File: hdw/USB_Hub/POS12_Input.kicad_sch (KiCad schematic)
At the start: 21 parts

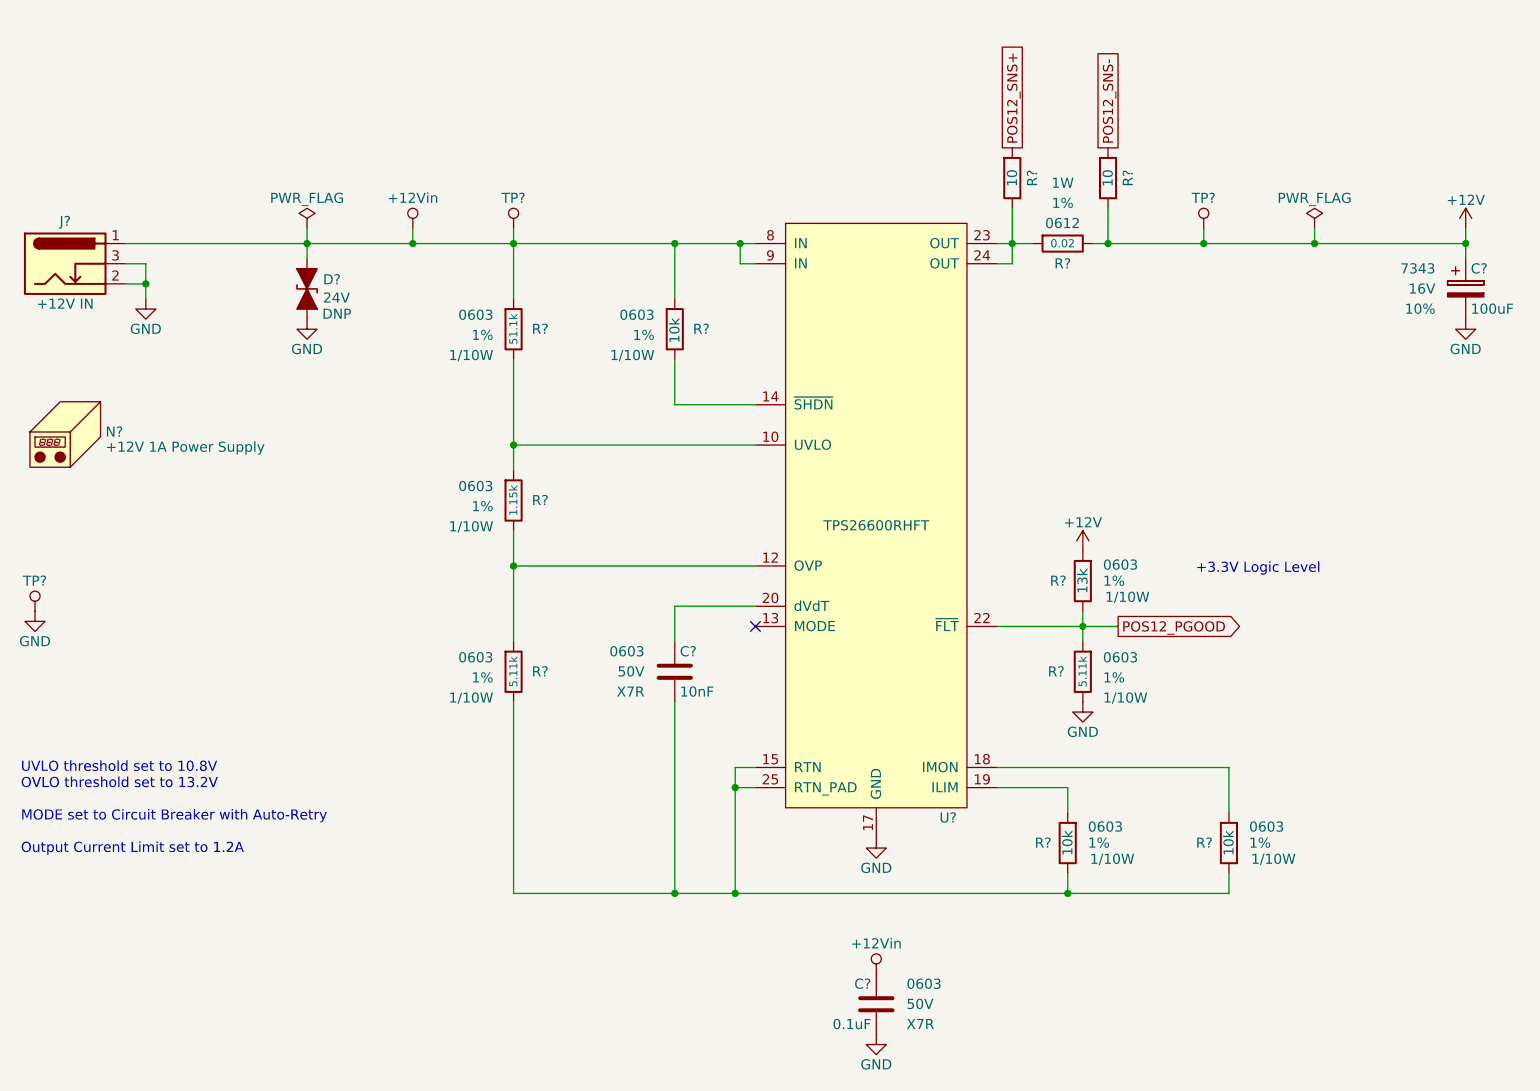
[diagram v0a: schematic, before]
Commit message: big restructuring, removed microcontroller and all telemtry
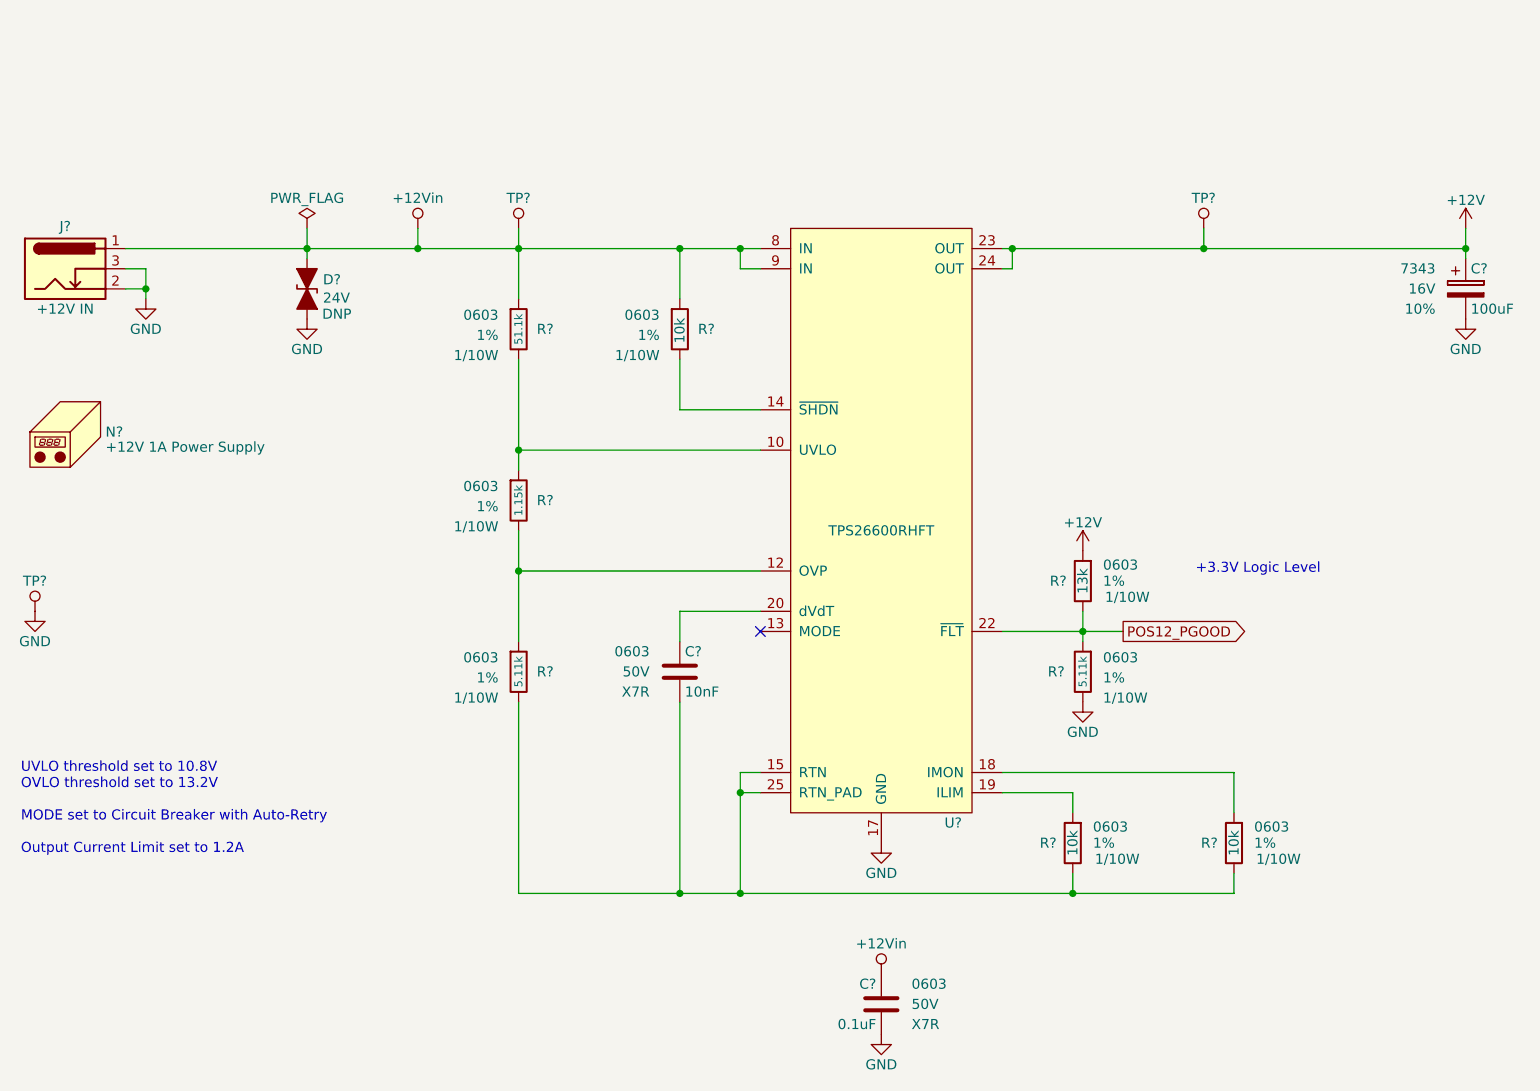
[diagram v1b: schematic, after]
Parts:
- removed R? (x2): 10, Resistors_SMD:R_0603, symbol Custom_Library:R_Custom
- removed R?: 0.02, Resistors_SMD:R_0612, symbol Custom_Library:R_Custom
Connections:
- net +12V: now also U?.23 (OUT), U?.24 (OUT)
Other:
- moved on the sheet: C?, J?, R?, TP?, U?

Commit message: fixed footprints, assigned digikey pns
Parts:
- R? (x3): Digi-Key PN (none) -> 541-10.0KHCT-ND
- R?: Digi-Key PN (none) -> 541-1.15KHCT-ND
- R?: Digi-Key PN (none) -> 541-13.0KHCT-ND
- R? (x2): Digi-Key PN (none) -> 541-5.11KHCT-ND
- R?: Digi-Key PN (none) -> 541-3009-1-ND
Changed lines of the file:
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@@
       (effects (font (size 1.27 1.27)) (justify left))
     )
-    (property "Digi-Key PN" "" (at 111.76 50.8 0)
+    (property "Digi-Key PN" "541-10.0KHCT-ND" (at 111.76 50.8 0)
       (effects (font (size 1.524 1.524)) hide)
     )
@@
       (effects (font (size 1.27 1.27)) (justify left))
     )
-    (property "Digi-Key PN" "" (at 91.44 72.39 0)
+    (property "Digi-Key PN" "541-1.15KHCT-ND" (at 91.44 72.39 0)
       (effects (font (size 1.524 1.524)) hide)
     )
@@
       (effects (font (size 1.27 1.27)) (justify left))
     )
-    (property "Digi-Key PN" "" (at 176.53 115.57 0)
+    (property "Digi-Key PN" "541-10.0KHCT-ND" (at 176.53 115.57 0)
       (effects (font (size 1.524 1.524)) hide)
     )
@@
       (effects (font (size 1.27 1.27)) (justify left))
     )
-    (property "Digi-Key PN" "" (at 170.18 92.71 0)
+    (property "Digi-Key PN" "541-13.0KHCT-ND" (at 170.18 92.71 0)
       (effects (font (size 1.27 1.27)) hide)
     )
@@
       (effects (font (size 1.27 1.27)) (justify left))
     )
-    (property "Digi-Key PN" "" (at 91.44 93.98 0)
+    (property "Digi-Key PN" "541-5.11KHCT-ND" (at 91.44 93.98 0)
       (effects (font (size 1.524 1.524)) hide)
     )
@@
       (effects (font (size 1.27 1.27)) (justify left))
     )
-    (property "Digi-Key PN" "" (at 196.85 115.57 0)
+    (property "Digi-Key PN" "541-10.0KHCT-ND" (at 196.85 115.57 0)
       (effects (font (size 1.524 1.524)) hide)
     )
@@
       (effects (font (size 1.27 1.27)) (justify left))
     )
-    (property "Digi-Key PN" "" (at 91.44 50.8 0)
+    (property "Digi-Key PN" "541-3009-1-ND" (at 91.44 50.8 0)
       (effects (font (size 1.524 1.524)) hide)
     )
@@
       (effects (font (size 1.27 1.27)) (justify left))
     )
-    (property "Digi-Key PN" "" (at 177.8 93.98 0)
+    (property "Digi-Key PN" "541-5.11KHCT-ND" (at 177.8 93.98 0)
       (effects (font (size 1.524 1.524)) hide)
     )
